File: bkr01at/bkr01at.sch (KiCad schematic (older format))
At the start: 1 part, among them U1 nRF52832-QFAB

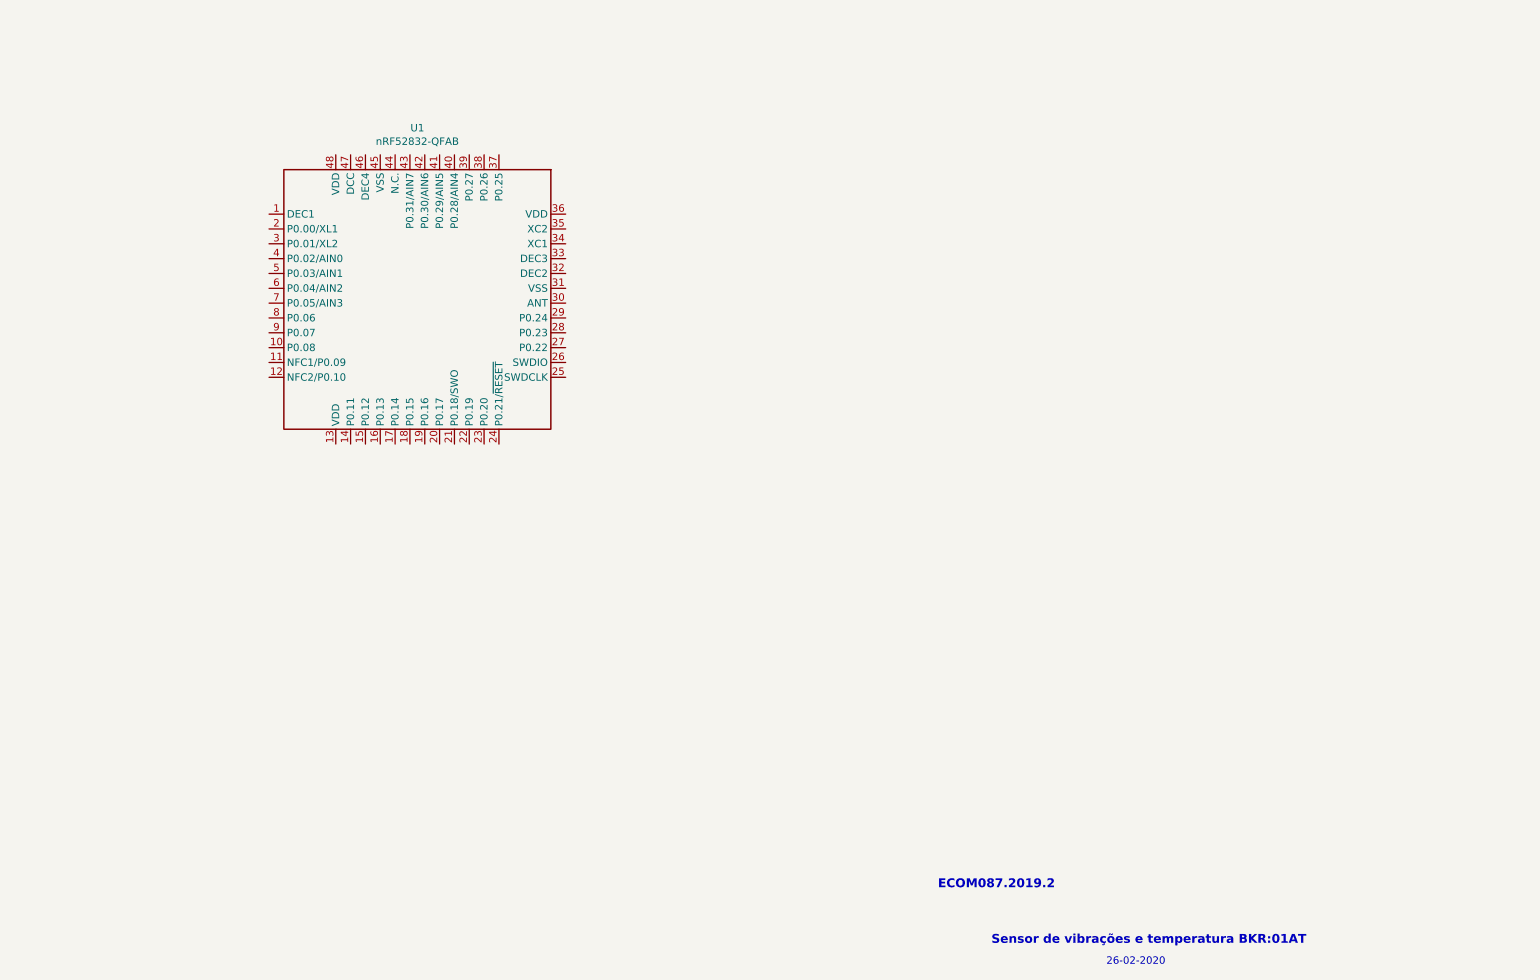
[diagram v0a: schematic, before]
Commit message: Finalizando esquemático. Começando PCB.
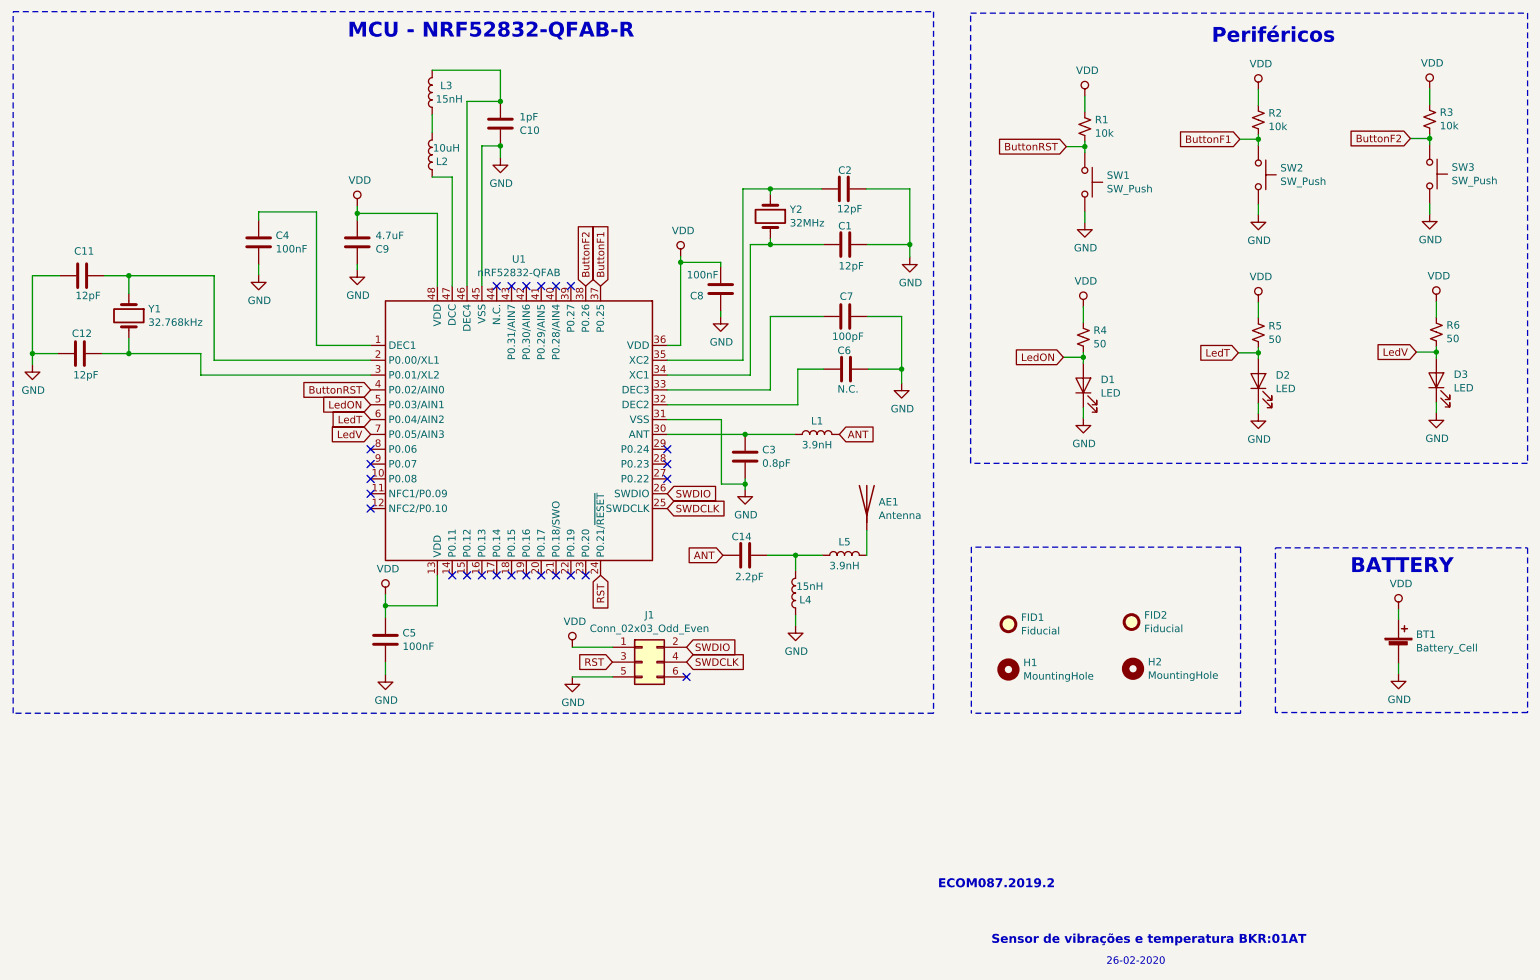
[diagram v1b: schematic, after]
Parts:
- added AE1: Antenna, antena_ble:2450AT18B100, symbol Device:Antenna
- added BT1: Battery_Cell, Battery:Battery_CR1225, symbol Device:Battery_Cell
- added C1, C11, C12, C2: 12pF, Capacitor_SMD:C_0402_1005Metric, symbol Device:C
- added C10: 1pF, Capacitor_SMD:C_0402_1005Metric, symbol Device:C
- added C14: 2.2pF, Capacitor_SMD:C_0402_1005Metric, symbol Device:C
- added C3: 0.8pF, Capacitor_SMD:C_0402_1005Metric, symbol Device:C
- added C4, C5, C8: 100nF, Capacitor_SMD:C_0402_1005Metric, symbol Device:C
- added C6: N.C., Capacitor_SMD:C_0402_1005Metric, symbol Device:C
- added C7: 100pF, Capacitor_SMD:C_0402_1005Metric, symbol Device:C
- added C9: 4.7uF, Capacitor_SMD:C_0402_1005Metric, symbol Device:C
- added D1, D2, D3: LED, LED_SMD:LED_0603_1608Metric, symbol Device:LED
- added FID1, FID2: Fiducial, Fiducial:Fiducial_0.5mm_Mask1.5mm, symbol Mechanical:Fiducial
- added H1, H2: MountingHole, MountingHole:MountingHole_3.2mm_M3, symbol Mechanical:MountingHole
- added J1: Conn_02x03_Odd_Even, Connector:Tag-Connect_TC2030-IDC-NL_2x03_P1.27mm_Vertical, symbol Connector_Generic:Conn_02x03_Odd_Even
- added L1, L5: 3.9nH, Inductor_SMD:L_0402_1005Metric, symbol Device:L
- added L2: 10uH, Inductor_SMD:L_0402_1005Metric, symbol Device:L
- added L3, L4: 15nH, Inductor_SMD:L_0402_1005Metric, symbol Device:L
- added R1, R2, R3: 10k, Resistor_SMD:R_0402_1005Metric, symbol Device:R_Small_US
- added R4, R5, R6: 50, Resistor_SMD:R_0402_1005Metric, symbol Device:R_Small_US
- added SW1, SW2, SW3: SW_Push, Button_Switch_SMD:SW_MEC_5GSH9, symbol Switch:SW_Push
- added Y1: 32.768kHz, Crystal:Crystal_SMD_3215-2Pin_3.2x1.5mm, symbol Device:Crystal
- added Y2: 32MHz, Crystal:Crystal_SMD_2016-4Pin_2.0x1.6mm, symbol Device:Crystal
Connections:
- net at U1.1 (DEC1): now also C4.1
- net VDD: now reaches U1.13 (VDD)
- net VDD: now also U1.36 (VDD), U1.48 (VDD), BT1.1 (+), C5.1, C8.2, C9.2, J1.1 (Pin_1), R1.1, R2.1, R3.1, R4.1, R5.1, R6.1
- net at U1.2 (P0.00/XL1): now also C11.1, Y1.1
- net RST: now reaches U1.24 (P0.21/~RESET)
- net RST: now also J1.3 (Pin_3)
- net SWDCLK: now reaches U1.25 (SWDCLK)
- net SWDCLK: now also J1.4 (Pin_4)
- net SWDIO: now reaches U1.26 (SWDIO)
- net SWDIO: now also J1.2 (Pin_2)
- net at U1.3 (P0.01/XL2): now also C12.1, Y1.2
- net at U1.30 (ANT): now also C3.1, L1.1
- net GND: now reaches U1.31 (VSS)
- net GND: now also U1.45 (VSS), BT1.2 (-), C1.2, C10.1, C11.2, C12.2, C2.2, C3.2, C4.2, C5.2, C6.2, C7.2, C8.1, C9.1, D1.1 (K), D2.1 (K), D3.1 (K), J1.5 (Pin_5), L4.1, SW1.2, SW2.2, SW3.2
- net at U1.32 (DEC2): now also C6.1
- net at U1.33 (DEC3): now also C7.1
- net at U1.34 (XC1): now also C1.1, Y2.2
- net at U1.35 (XC2): now also C2.1, Y2.1
- net ButtonF1: now reaches U1.37 (P0.25)
- net ButtonF1: now also R2.2, SW2.1
- net ButtonF2: now reaches U1.38 (P0.26)
- net ButtonF2: now also R3.2, SW3.1
- net ButtonRST: now reaches U1.4 (P0.02/AIN0)
- net ButtonRST: now also R1.2, SW1.1
- net at U1.46 (DEC4): now also C10.2, L3.2
- net at U1.47 (DCC): now also L2.1
- net LedON: now reaches U1.5 (P0.03/AIN1)
- net LedON: now also D1.2 (A), R4.2
- net LedT: now reaches U1.6 (P0.04/AIN2)
- net LedT: now also D2.2 (A), R5.2
- net LedV: now reaches U1.7 (P0.05/AIN3)
- net LedV: now also D3.2 (A), R6.2
- new net: L2.2, L3.1
- new net: C14.2, L4.2, L5.1
- new net: AE1.1 (A), L5.2
- new net ANT: C14.1, L1.2
- no-connect marks 0 -> 25
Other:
- note added: "BATTERY"
- note added: "MCU - NRF52832-QFAB-R"
- note added: "Periféricos"
- moved on the sheet: U1

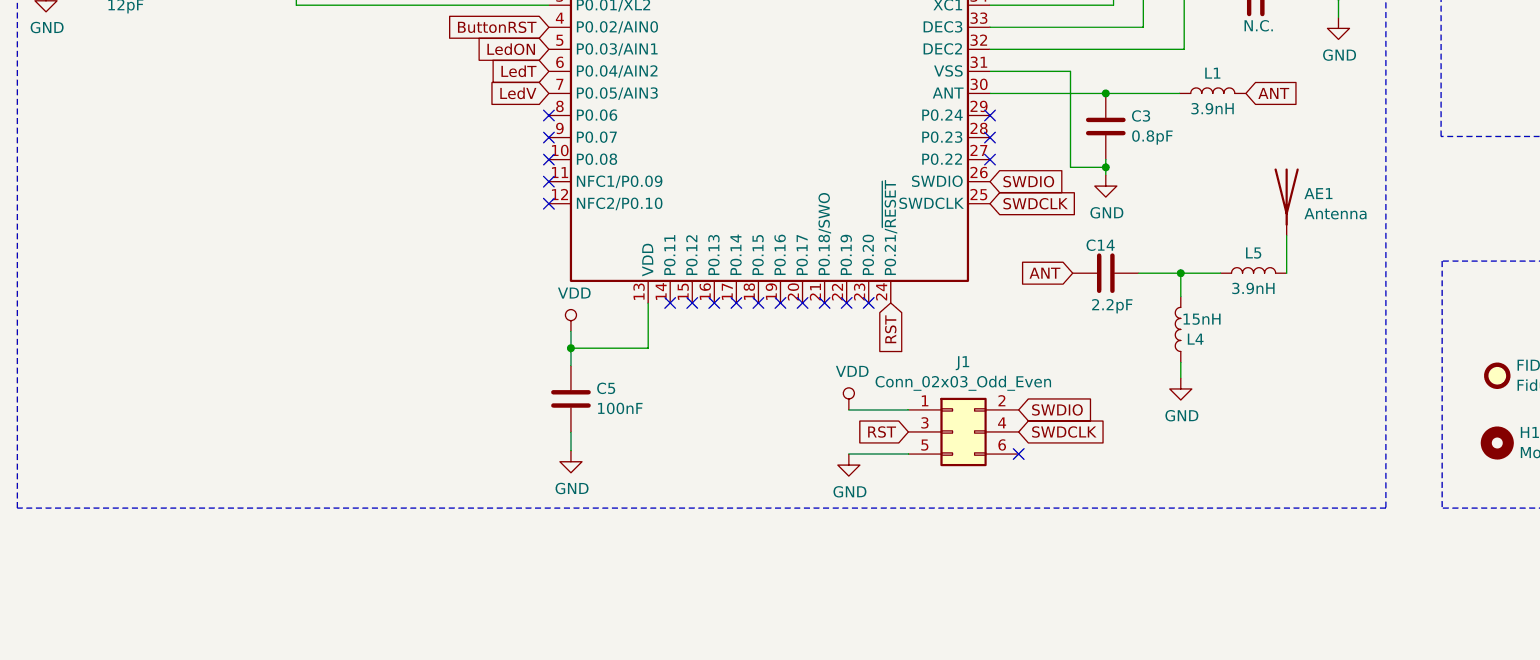
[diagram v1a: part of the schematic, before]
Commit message: Atualizando esquemático.
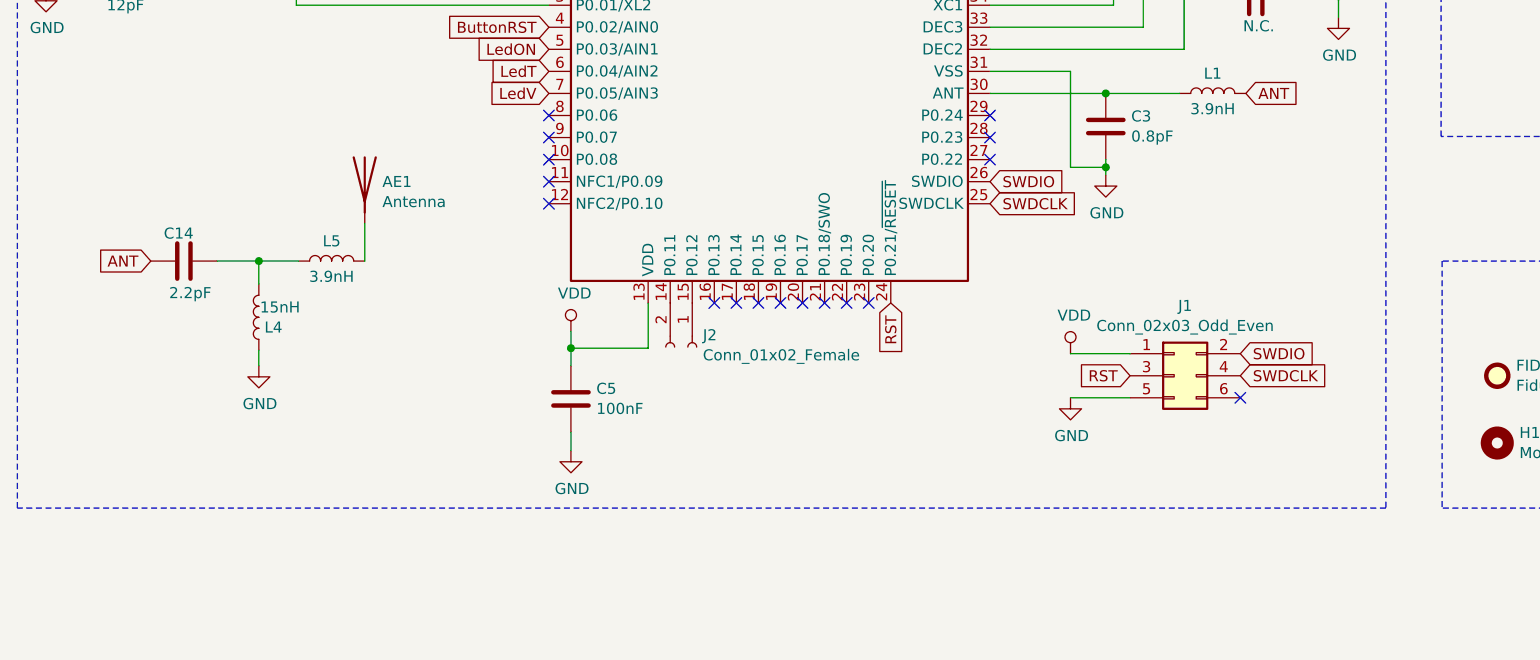
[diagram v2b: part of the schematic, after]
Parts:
- added J2: Conn_01x02_Female, Connector:Banana_Jack_2Pin, symbol Connector:Conn_01x02_Female
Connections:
- net at U1.14 (P0.11): now also J2.2 (Pin_2)
- net at U1.15 (P0.12): now also J2.1 (Pin_1)
- no-connect marks 25 -> 23
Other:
- moved on the sheet: AE1, C14, J1, L4, L5
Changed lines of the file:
@@
 L Device:C C14
 U 1 1 5E75BE65
-P 5700 4875
-F 0 "C14" V 5825 4831 50  0000 L CNN
-F 1 "2.2pF" V 5555 4750 50  0000 L CNN
-F 2 "Capacitor_SMD:C_0402_1005Metric" H 5738 4725 50  0001 C CNN
-F 3 "~" H 5700 4875 50  0001 C CNN
-	1    5700 4875
+P 1520 4820
+F 0 "C14" V 1645 4776 50  0000 L CNN
+F 1 "2.2pF" V 1375 4695 50  0000 L CNN
+F 2 "Capacitor_SMD:C_0402_1005Metric" H 1558 4670 50  0001 C CNN
+F 3 "~" H 1520 4820 50  0001 C CNN
+	1    1520 4820
 	0    -1   -1   0
 $EndComp
@@
 L Device:L L5
 U 1 1 5E76400C
-P 6370 4875
-F 0 "L5" V 6460 4875 50  0000 C CNN
-F 1 "3.9nH" V 6299 4875 50  0000 C CNN
-F 2 "Inductor_SMD:L_0402_1005Metric" H 6370 4875 50  0001 C CNN
-F 3 "~" H 6370 4875 50  0001 C CNN
-	1    6370 4875
+P 2190 4820
+F 0 "L5" V 2280 4820 50  0000 C CNN
+F 1 "3.9nH" V 2119 4820 50  0000 C CNN
+F 2 "Inductor_SMD:L_0402_1005Metric" H 2190 4820 50  0001 C CNN
+F 3 "~" H 2190 4820 50  0001 C CNN
+	1    2190 4820
 	0    -1   -1   0
 $EndComp
@@
 L Device:L L4
 U 1 1 5E76EC23
-P 6040 5130
-F 0 "L4" H 5933 5176 50  0000 L CNN
-F 1 "15nH" H 5853 5085 50  0000 L CNN
-F 2 "Inductor_SMD:L_0402_1005Metric" H 6040 5130 50  0001 C CNN
-F 3 "~" H 6040 5130 50  0001 C CNN
-	1    6040 5130
+P 1860 5075
+F 0 "L4" H 1753 5121 50  0000 L CNN
+F 1 "15nH" H 1673 5030 50  0000 L CNN
+F 2 "Inductor_SMD:L_0402_1005Metric" H 1860 5075 50  0001 C CNN
+F 3 "~" H 1860 5075 50  0001 C CNN
+	1    1860 5075
 	-1   0    0    1
 $EndComp
-Text GLabel 5550 4875 0    50   Input ~ 0
+Text GLabel 1370 4820 0    50   Input ~ 0
 ANT
 Wire Wire Line
-	5850 4875 6040 4875
-Wire Wire Line
-	6040 4980 6040 4875
-Connection ~ 6040 4875
-Wire Wire Line
-	6040 4875 6220 4875
+	1670 4820 1860 4820
+Wire Wire Line
+	1860 4925 1860 4820
+Connection ~ 1860 4820
+Wire Wire Line
+	1860 4820 2040 4820
 $Comp
 L power:GND #PWR0115
 U 1 1 5E779C31
-P 6040 5350
-F 0 "#PWR0115" H 6040 5100 50  0001 C CNN
-F 1 "GND" H 6045 5177 50  0000 C CNN
-F 2 "" H 6040 5350 50  0001 C CNN
-F 3 "" H 6040 5350 50  0001 C CNN
-	1    6040 5350
-	1    0    0    -1
-$EndComp
-Wire Wire Line
-	6040 5280 6040 5350
+P 1860 5295
+F 0 "#PWR0115" H 1860 5045 50  0001 C CNN
+F 1 "GND" H 1865 5122 50  0000 C CNN
+F 2 "" H 1860 5295 50  0001 C CNN
+F 3 "" H 1860 5295 50  0001 C CNN
+	1    1860 5295
+	1    0    0    -1
+$EndComp
+Wire Wire Line
+	1860 5225 1860 5295
 $Comp
 L Device:Antenna AE1
 U 1 1 5E77DED0
-P 6520 4505
-F 0 "AE1" H 6600 4494 50  0000 L CNN
-F 1 "Antenna" H 6600 4403 50  0000 L CNN
-F 2 "antena_ble:2450AT18B100" H 6520 4505 50  0001 C CNN
-F 3 "~" H 6520 4505 50  0001 C CNN
-	1    6520 4505
-	1    0    0    -1
-$EndComp
-Wire Wire Line
-	6520 4875 6520 4705
+P 2340 4450
+F 0 "AE1" H 2420 4439 50  0000 L CNN
+F 1 "Antenna" H 2420 4348 50  0000 L CNN
+F 2 "antena_ble:2450AT18B100" H 2340 4450 50  0001 C CNN
+F 3 "~" H 2340 4450 50  0001 C CNN
+	1    2340 4450
+	1    0    0    -1
+$EndComp
+Wire Wire Line
+	2340 4820 2340 4650
 $Comp
 L Switch:SW_Push SW3
@@
 L Connector_Generic:Conn_02x03_Odd_Even J1
 U 1 1 5E9302B4
-P 5005 5595
-F 0 "J1" H 5055 5912 50  0000 C CNN
-F 1 "Conn_02x03_Odd_Even" H 5055 5821 50  0000 C CNN
-F 2 "Connector:Tag-Connect_TC2030-IDC-NL_2x03_P1.27mm_Vertical" H 5005 5595 50  0001 C CNN
-F 3 "~" H 5005 5595 50  0001 C CNN
-	1    5005 5595
+P 6010 5340
+F 0 "J1" H 6060 5657 50  0000 C CNN
+F 1 "Conn_02x03_Odd_Even" H 6060 5566 50  0000 C CNN
+F 2 "Connector:Tag-Connect_TC2030-IDC-NL_2x03_P1.27mm_Vertical" H 6010 5340 50  0001 C CNN
+F 3 "~" H 6010 5340 50  0001 C CNN
+	1    6010 5340
 	1    0    0    -1
 $EndComp
 Text GLabel 4725 5010 3    50   Input ~ 0
 RST
-Text GLabel 4805 5595 0    50   Input ~ 0
+Text GLabel 5810 5340 0    50   Input ~ 0
 RST
 Text GLabel 5175 4460 2    50   Input ~ 0
 SWDIO
-Text GLabel 5305 5495 2    50   Input ~ 0
+Text GLabel 6310 5240 2    50   Input ~ 0
 SWDIO
-Text GLabel 5305 5595 2    50   Input ~ 0
+Text GLabel 6310 5340 2    50   Input ~ 0
 SWDCLK
 Text GLabel 5175 4560 2    50   Input ~ 0
@@
 L power:GND #PWR0128
 U 1 1 5E957922
-P 4535 5695
-F 0 "#PWR0128" H 4535 5445 50  0001 C CNN
-F 1 "GND" H 4540 5522 50  0000 C CNN
-F 2 "" H 4535 5695 50  0001 C CNN
-F 3 "" H 4535 5695 50  0001 C CNN
-	1    4535 5695
+P 5540 5440
+F 0 "#PWR0128" H 5540 5190 50  0001 C CNN
+F 1 "GND" H 5545 5267 50  0000 C CNN
+F 2 "" H 5540 5440 50  0001 C CNN
+F 3 "" H 5540 5440 50  0001 C CNN
+	1    5540 5440
 	1    0    0    -1
 $EndComp
@@
 L power:VDD #PWR0129
 U 1 1 5E968E7B
-P 4535 5495
-F 0 "#PWR0129" H 4535 5345 50  0001 C CNN
-F 1 "VDD" H 4552 5668 50  0000 C CNN
-F 2 "" H 4535 5495 50  0001 C CNN
-F 3 "" H 4535 5495 50  0001 C CNN
-	1    4535 5495
-	1    0    0    -1
-$EndComp
-Wire Wire Line
-	4805 5495 4535 5495
-NoConn ~ 5305 5695
-NoConn ~ 3725 5010
-NoConn ~ 3825 5010
-Wire Wire Line
-	4805 5695 4535 5695
+P 5540 5240
+F 0 "#PWR0129" H 5540 5090 50  0001 C CNN
+F 1 "VDD" H 5557 5413 50  0000 C CNN
+F 2 "" H 5540 5240 50  0001 C CNN
+F 3 "" H 5540 5240 50  0001 C CNN
+	1    5540 5240
+	1    0    0    -1
+$EndComp
+Wire Wire Line
+	5810 5240 5540 5240
+NoConn ~ 6310 5440
+Wire Wire Line
+	5810 5440 5540 5440
 NoConn ~ 4425 5010
 $Comp
@@
 Wire Notes Line
 	7225 4820 7225 5940
+$Comp
+L Connector:Conn_01x02_Female J2
+U 1 1 5E5C2C6B
+P 3825 5210
+F 0 "J2" V 3771 5258 50  0000 L CNN
+F 1 "Conn_01x02_Female" V 3862 5258 50  0000 L CNN
+F 2 "Connector:Banana_Jack_2Pin" H 3825 5210 50  0001 C CNN
+F 3 "~" H 3825 5210 50  0001 C CNN
+	1    3825 5210
+	0    1    1    0
+$EndComp
 $EndSCHEMATC
